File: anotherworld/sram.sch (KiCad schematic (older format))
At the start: 5 parts

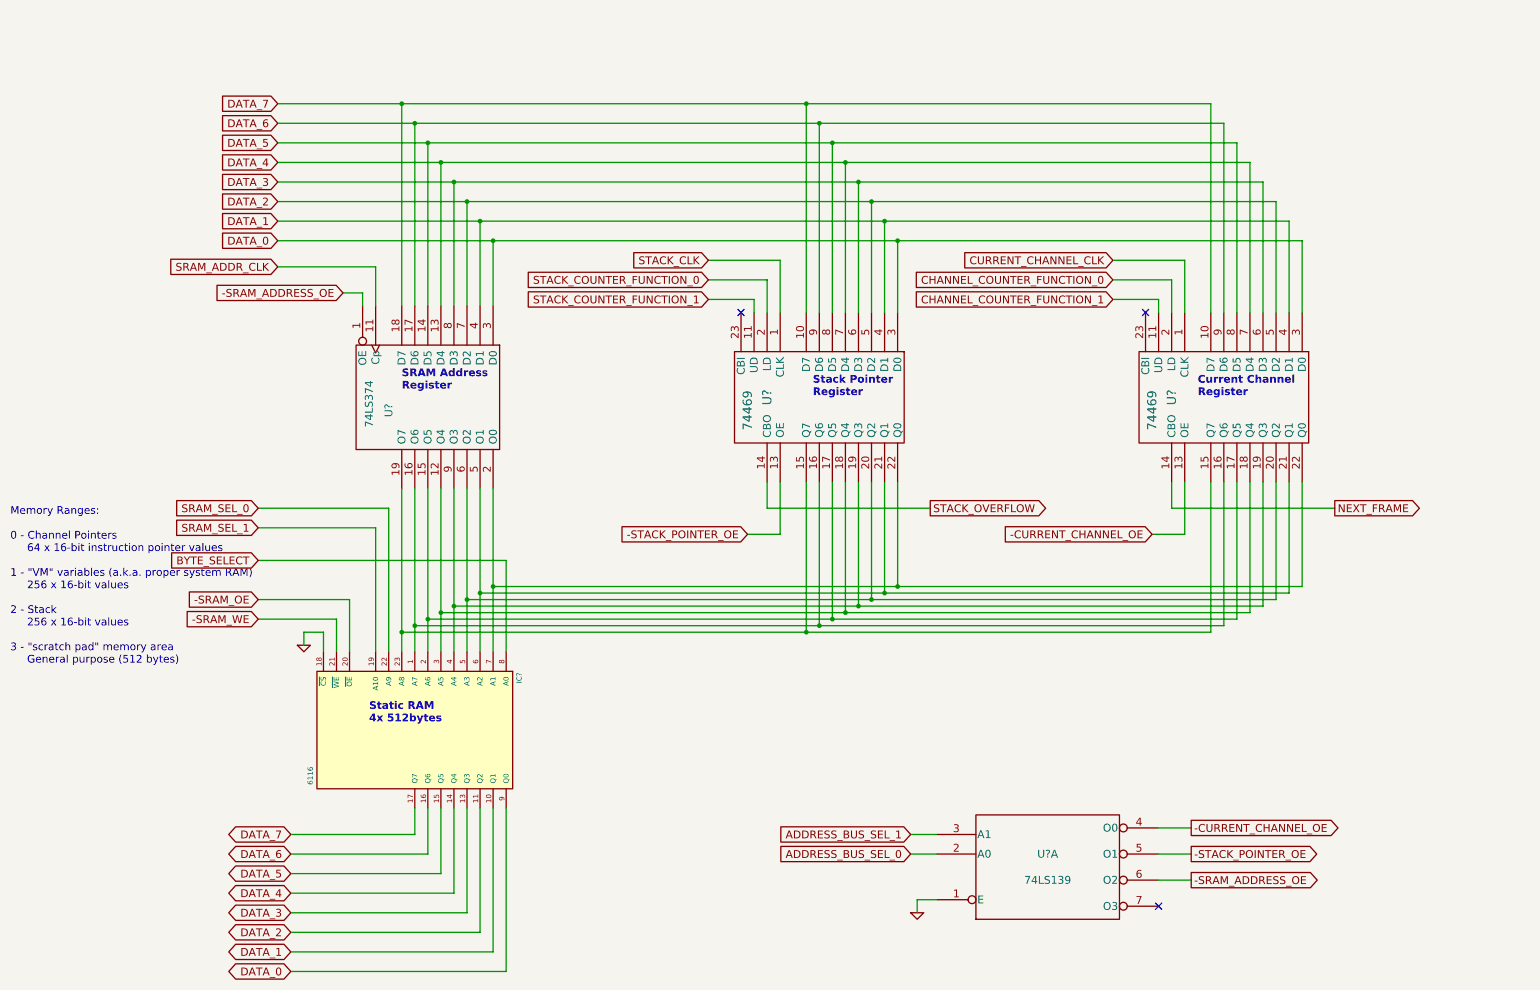
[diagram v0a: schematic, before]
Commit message: weekly workshop update
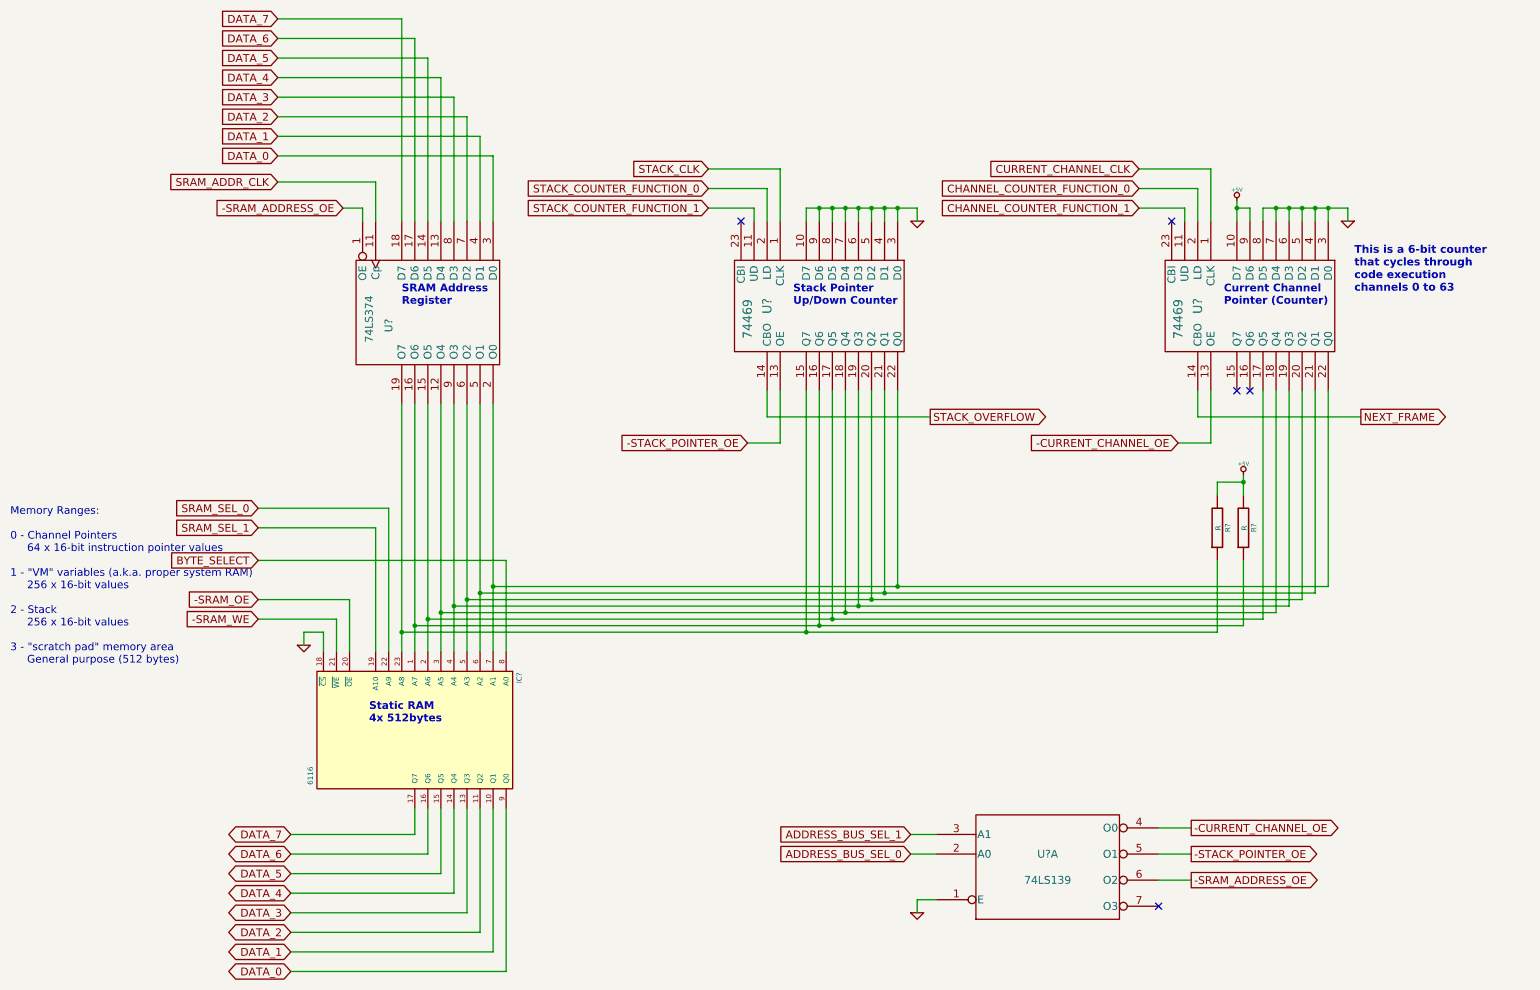
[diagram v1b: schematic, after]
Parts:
- added R? (x2): R, ~, symbol R
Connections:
- net DATA_0: no longer U?.3 (D0), U?.3 (D0)
- net DATA_1: no longer U?.4 (D1), U?.4 (D1)
- net DATA_2: no longer U?.5 (D2), U?.5 (D2)
- net DATA_3: no longer U?.6 (D3), U?.6 (D3)
- net DATA_4: no longer U?.7 (D4), U?.7 (D4)
- net DATA_5: no longer U?.8 (D5), U?.8 (D5)
- net DATA_6: no longer U?.9 (D6), U?.9 (D6)
- net DATA_7: no longer U?.10 (D7), U?.10 (D7)
- net GND: now also U?.10 (D7), U?.3 (D0), U?.3 (D0), U?.4 (D1), U?.4 (D1), U?.5 (D2), U?.5 (D2), U?.6 (D3), U?.6 (D3), U?.7 (D4), U?.7 (D4), U?.8 (D5), U?.8 (D5), U?.9 (D6)
- net at IC?.1 (A7), U?.16 (O6), U?.16 (Q6): now also R?.1; no longer U?.16 (Q6)
- net at IC?.23 (A8), U?.15 (Q7), U?.19 (O7): now also R?.1; no longer U?.15 (Q7)
- new net +5V: R?.2, R?.2, U?.10 (D7), U?.9 (D6)
- no-connect marks 3 -> 5
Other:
- note added: "Current Channel\nPointer (Counter)"
- note added: "Stack Pointer\nUp/Down Counter"
- note added: "This is a 6-bit counter\nthat cycles through\ncode execution\nchannels 0 to 63"
- note removed: "Current Channel\nRegister"
- note removed: "Stack Pointer\nRegister"
- moved on the sheet: U?
